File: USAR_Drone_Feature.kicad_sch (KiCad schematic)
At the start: 48 parts, among them J1 DB128L-5.08-2P-BK-S, J2 DB128L-5.08-2P-BK-S, J3 Conn_02x04_Odd_Even, J4 Conn_01x04_Socket, J5 Conn_01x04_Socket, J6 Conn_01x04_Socket, SW1 TS-1088-AR02016, SW2 TS-1088-AR02016, U1 ESP32-S3-WROOM-1(N16R8)

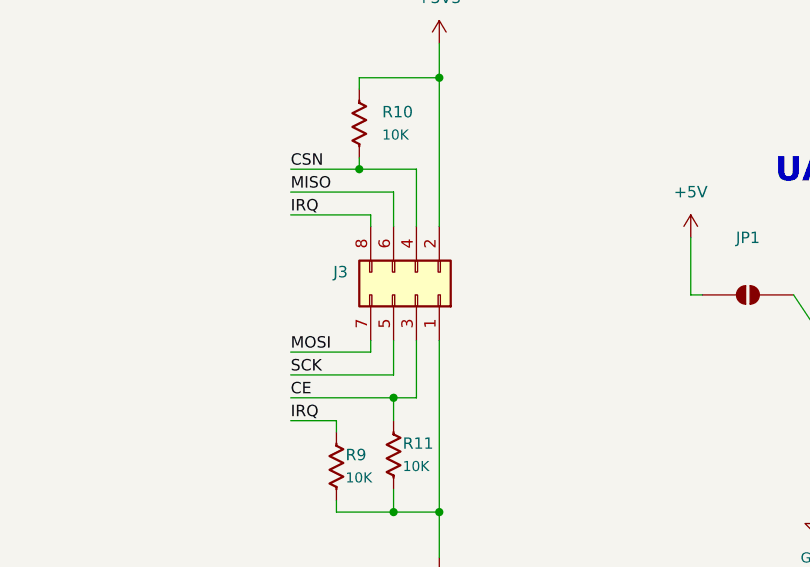
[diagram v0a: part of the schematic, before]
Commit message: ajuste de agujeros
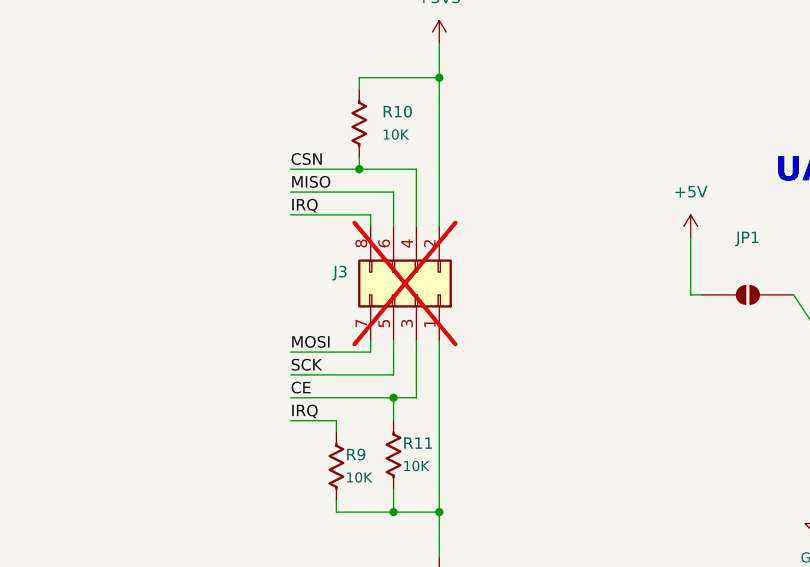
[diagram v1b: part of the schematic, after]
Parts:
- J3: now not fitted
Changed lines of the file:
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@@
 		(on_board yes)
 		(in_pos_files yes)
-		(dnp no)
+		(dnp yes)
 		(property "Reference" "J3"
 			(at 191.77 226.0599 90)
